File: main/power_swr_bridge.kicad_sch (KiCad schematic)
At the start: 15 parts, among them J7 Conn_Coaxial

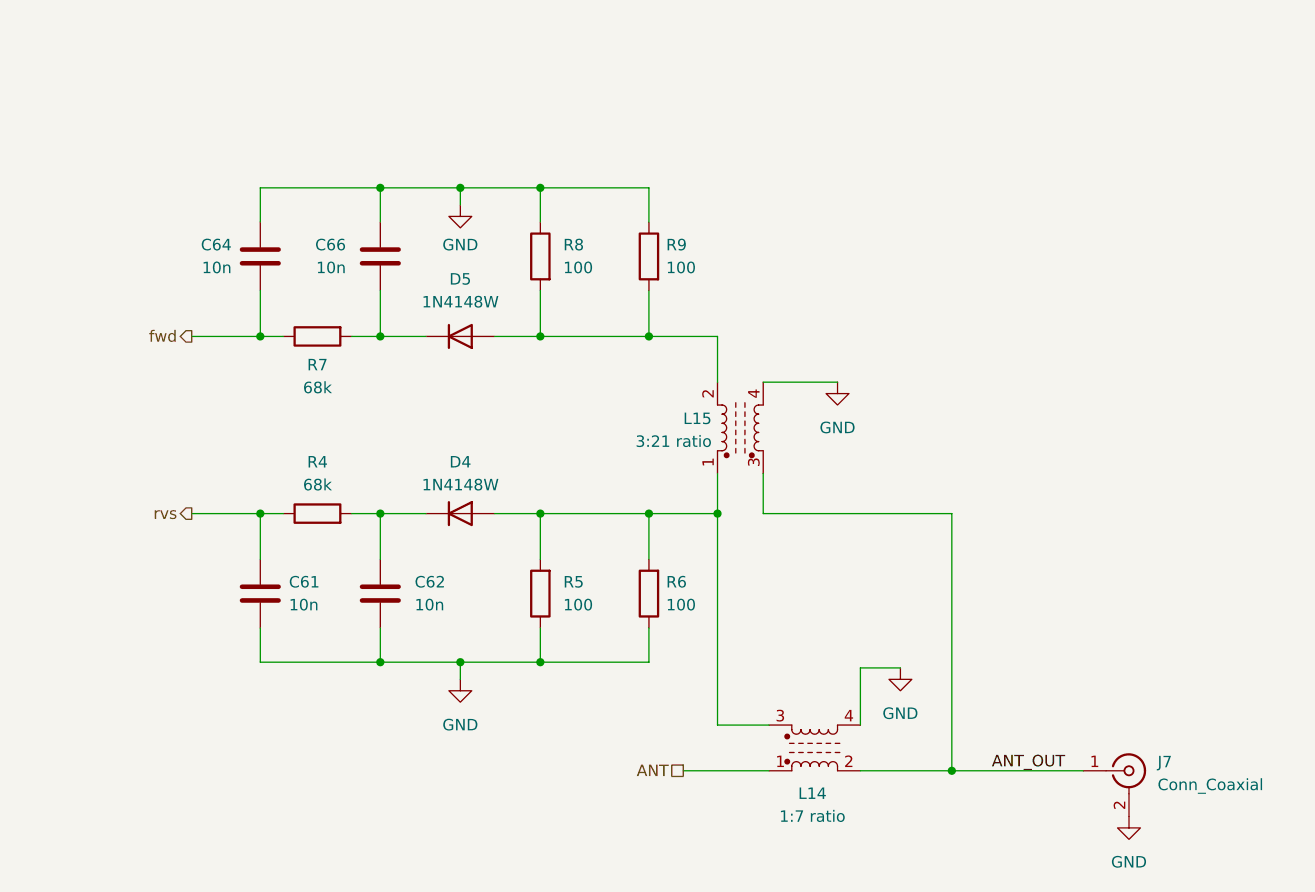
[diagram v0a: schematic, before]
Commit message: swr bridge mirrored for better look
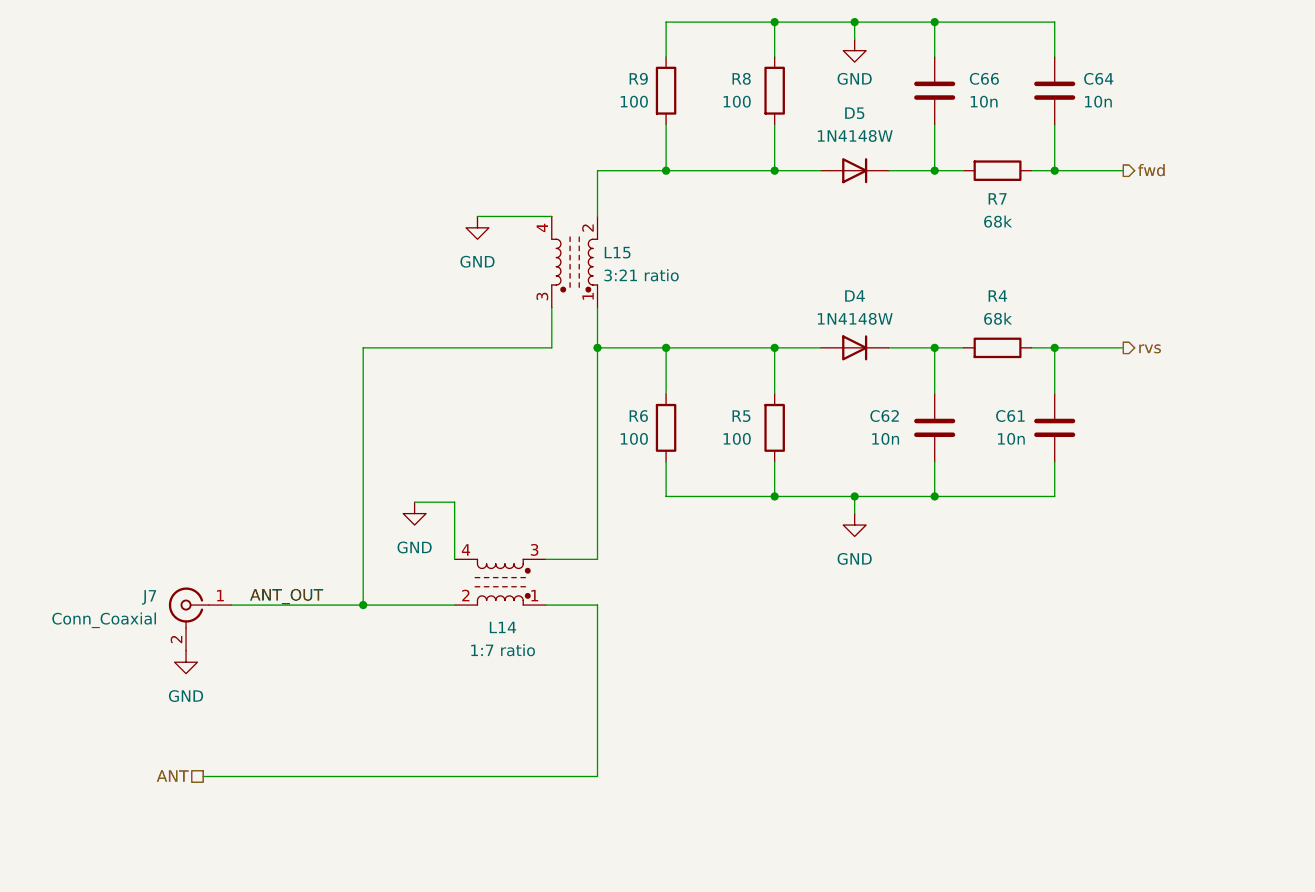
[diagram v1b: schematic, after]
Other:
- moved on the sheet: C61, C62, C64, C66, D4, D5, J7, L14, L15, R4, R5, R6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
